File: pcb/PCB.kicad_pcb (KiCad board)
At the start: 4 copper layers, 29.2 x 51.1 mm, 35 parts, among them J1 Conn_01x15, J2 USB_C_Receptacle_USB2.0, J3 Conn_01x15, J4 TC2030, J5 Conn_01x04, SW1 SW_Push, SW2 SW_Push, U1 SN65HVD230, U2 AMS1117-3.3, U3 STM32F103C8T6, Y1 8MHz

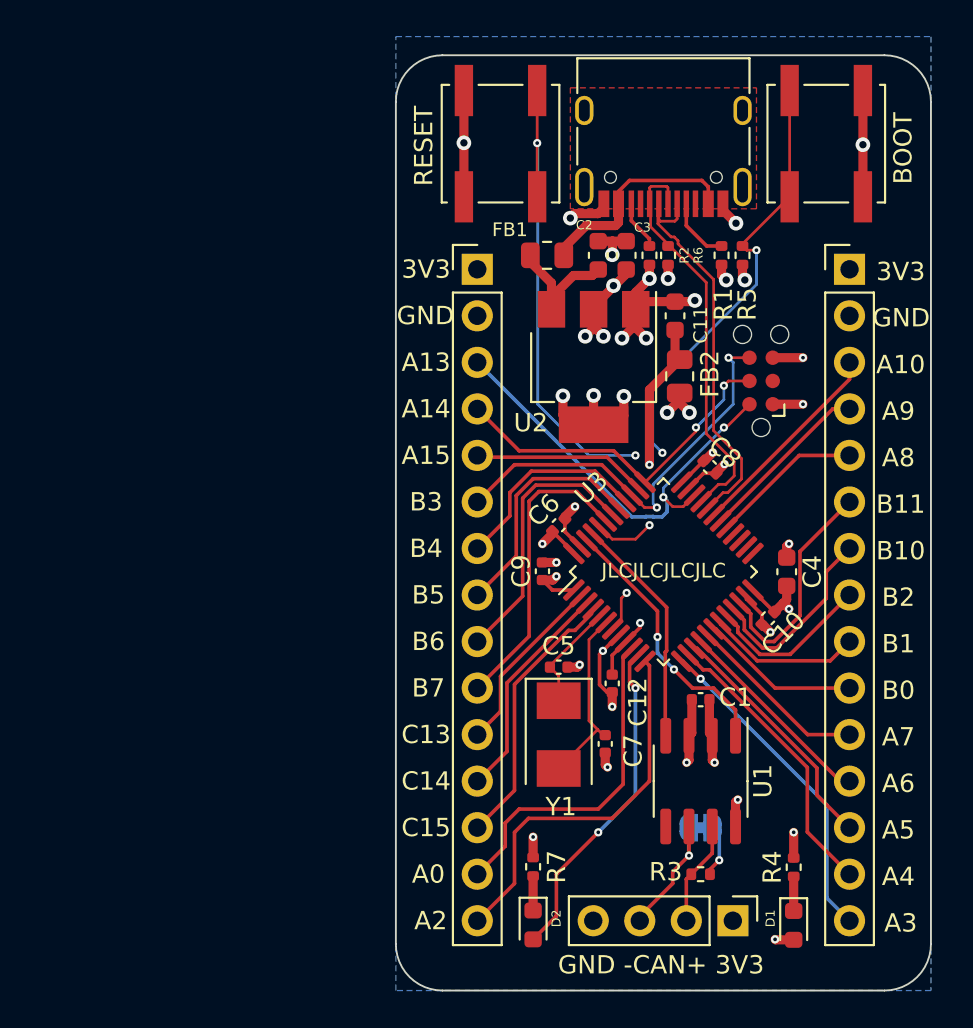
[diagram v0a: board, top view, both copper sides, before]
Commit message: Added circuit things
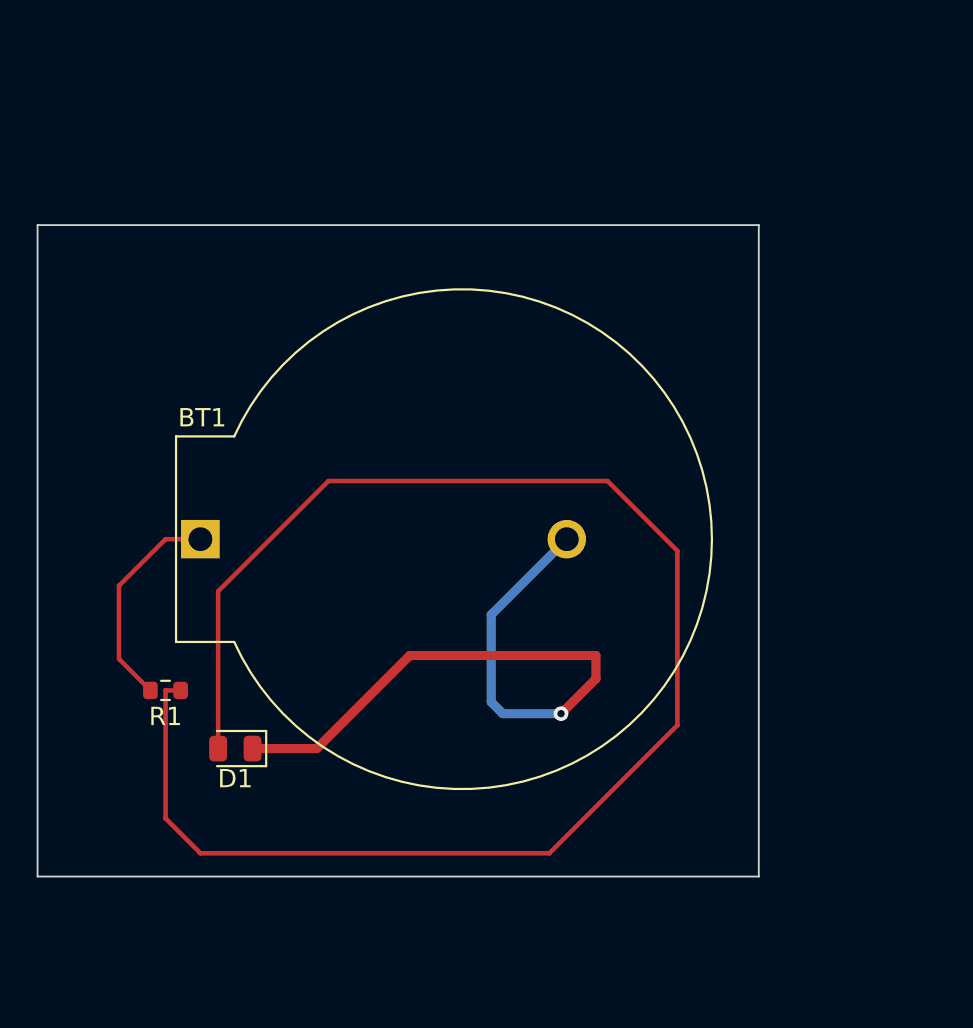
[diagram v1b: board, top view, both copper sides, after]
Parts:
- removed C1, C10, C12, C6, C8, C9: 100n, Capacitor_SMD:C_0402_1005Metric
- removed C11, C2, C3: 1u, Capacitor_SMD:C_0603_1608Metric
- removed C4: 4u7, Capacitor_SMD:C_0603_1608Metric
- removed C5, C7: 30p, Capacitor_SMD:C_0402_1005Metric
- removed D2: BLUE, LED_SMD:LED_0603_1608Metric
- removed FB1, FB2: 100R@100MHz, Resistor_SMD:R_0805_2012Metric
- removed J1, J3: Conn_01x15, Connector_PinHeader_2.54mm:PinHeader_1x15_P2.54mm_Vertical
- removed J2: USB_C_Receptacle_USB2.0, Connector_USB:USB_C_Receptacle_HRO_TYPE-C-31-M-12
- removed J4: TC2030, Connector:Tag-Connect_TC2030-IDC-NL_2x03_P1.27mm_Vertical
- removed J5: Conn_01x04, Connector_PinHeader_2.54mm:PinHeader_1x04_P2.54mm_Vertical
- removed JP1: SolderJumper_Bridged, Jumper:SolderJumper-2_P1.3mm_Bridged_RoundedPad1.0x1.5mm
- removed R2, R5: 5k1, Resistor_SMD:R_0402_1005Metric
- removed R3: 120R, Resistor_SMD:R_0402_1005Metric
- removed R4, R6, R7: 1k5, Resistor_SMD:R_0402_1005Metric
- removed SW1, SW2: SW_Push, Button_Switch_SMD:SW_Push_1P1T_NO_CK_KSC7xxJ
- removed U1: SN65HVD230, Package_SO:SOIC-8_3.9x4.9mm_P1.27mm
- removed U2: AMS1117-3.3, Package_TO_SOT_SMD:SOT-223-3_TabPin2
- removed U3: STM32F103C8T6, Package_QFP:LQFP-48_7x7mm_P0.5mm
- removed Y1: 8MHz, Crystal:Crystal_SMD_5032-2Pin_5.0x3.2mm
- added BT1: 12V, Battery:BatteryHolder_ComfortableElectronic_CH273-2450_1x2450, F.Cu at (122.0, 103.6)
- D1: value YELLOW -> LED; footprint LED_SMD:LED_0603_1608Metric -> LED_SMD:LED_0805_2012Metric
- R1: value 5k1 -> R; footprint Resistor_SMD:R_0402_1005Metric -> Resistor_SMD:R_0603_1608Metric
- moved R1 38.5 mm to (120.1, 111.9), turned to 180 degrees
- moved D1 32.0 mm to (124.0, 115.1), turned to 180 degrees
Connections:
- D1 pad 1: Net-(D1-Pad1) -> GND
- D1 pad 2: +3V3 -> Net-(D1-Pad2)
- R1 pad 1: Net-(J2-PadA5) -> Net-(D1-Pad2)
- R1 pad 2: GND -> battery positive
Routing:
- net Net-(D1-Pad2): track 0.00 -> 86.7 mm
- net +3V3: track 44.0 -> 0.00 mm, vias 18 -> 0
- net /NRST: track 35.9 -> 0.00 mm, vias 3 -> 0
- net /BOOT0: track 31.5 -> 0.00 mm, vias 3 -> 0
- net SWDIO: track 24.1 -> 0.00 mm, vias 2 -> 0
- net SWO: track 22.9 -> 0.00 mm, vias 2 -> 0
- net USB_D-: track 21.7 -> 0.00 mm
- net USB_D+: track 21.3 -> 0.00 mm
- net PA2: track 20.8 -> 0.00 mm
- net +3.3VA: track 20.2 -> 0.00 mm, vias 2 -> 0
- net SWCLK: track 19.4 -> 0.00 mm, vias 2 -> 0
- net PA0: track 18.4 -> 0.00 mm
- net /LED_STAT: track 18.2 -> 0.00 mm, vias 2 -> 0
- net PA3: track 18.0 -> 0.00 mm, vias 1 -> 0
- net PB7: track 16.5 -> 0.00 mm
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- removed copper zone on In2.Cu, net +3V3
- removed copper zone on B.Cu, net GND
- removed copper zone on In1.Cu, net GND
- removed copper zone on F.Cu, net unconnected-(J2-PadS1)
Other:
- board size 29.2 x 51.1 mm -> 39.4 x 35.6 mm
- board text removed: "3V3"
- board text removed: "3V3 +CAN- GND"
- board text removed: "A0"
- board text removed: "A10"
- board text removed: "A13"
- board text removed: "A14"
- board text removed: "A15"
- board text removed: "A2"
- board text removed: "A3"
- board text removed: "A4"
- board text removed: "A5"
- board text removed: "A6"
- board text removed: "A7"
- board text removed: "A8"
- board text removed: "A9"
- board text removed: "B0"
- board text removed: "B1"
- board text removed: "B10"
- board text removed: "B11"
- board text removed: "B2"
- board text removed: "B3"
- board text removed: "B4"
- board text removed: "B5"
- board text removed: "B6"
- board text removed: "B7"
- board text removed: "BOOT"
- board text removed: "C13"
- board text removed: "C14"
- board text removed: "C15"
- board text removed: "CAN TERM"
- board text removed: "GND"
- board text removed: "GND -CAN+ 3V3"
- board text removed: "JLCJLCJLCJLC"
- board text removed: "RESET"
- board text removed: "Rev 1"
- board text removed: "STM32F103 CAN/USB-C Jack LeFevre July 2022"
- board text removed: "SWCLK"
- board text removed: "SWDIO"
- board text removed: "SWO"
